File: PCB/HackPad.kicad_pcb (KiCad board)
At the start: 2 copper layers, 61.5 x 94 mm, 34 parts, among them SW1 SW_Push, SW10 RotaryEncoder, SW2 SW_Push, SW3 SW_Push, SW4 SW_Push, SW5 SW_Push, SW6 SW_Push, SW7 SW_Push, SW8 SW_Push, SW9 SW_Push, U1 MOUDLE-SEEEDUINO-XIAO, U2 ER_OLEDM0.91_1x-I2C

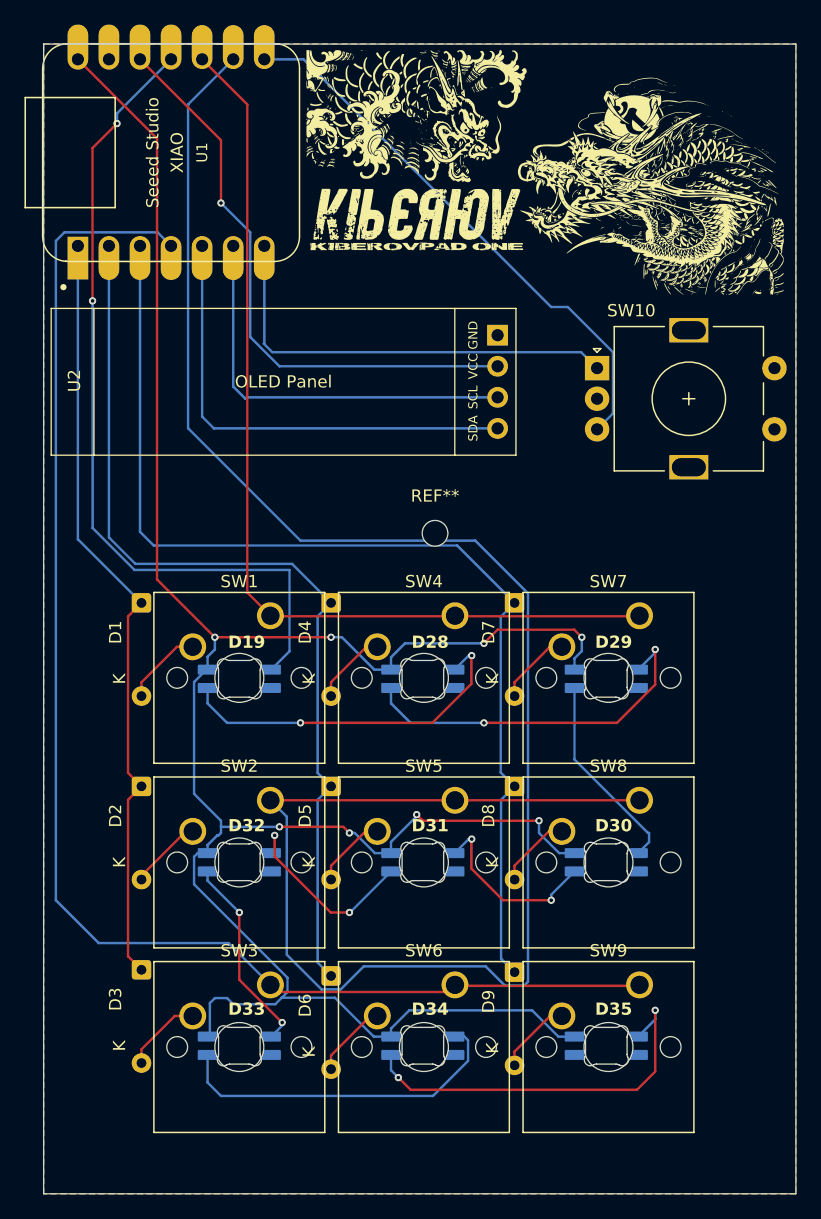
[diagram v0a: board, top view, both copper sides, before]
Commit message: changed pcb design
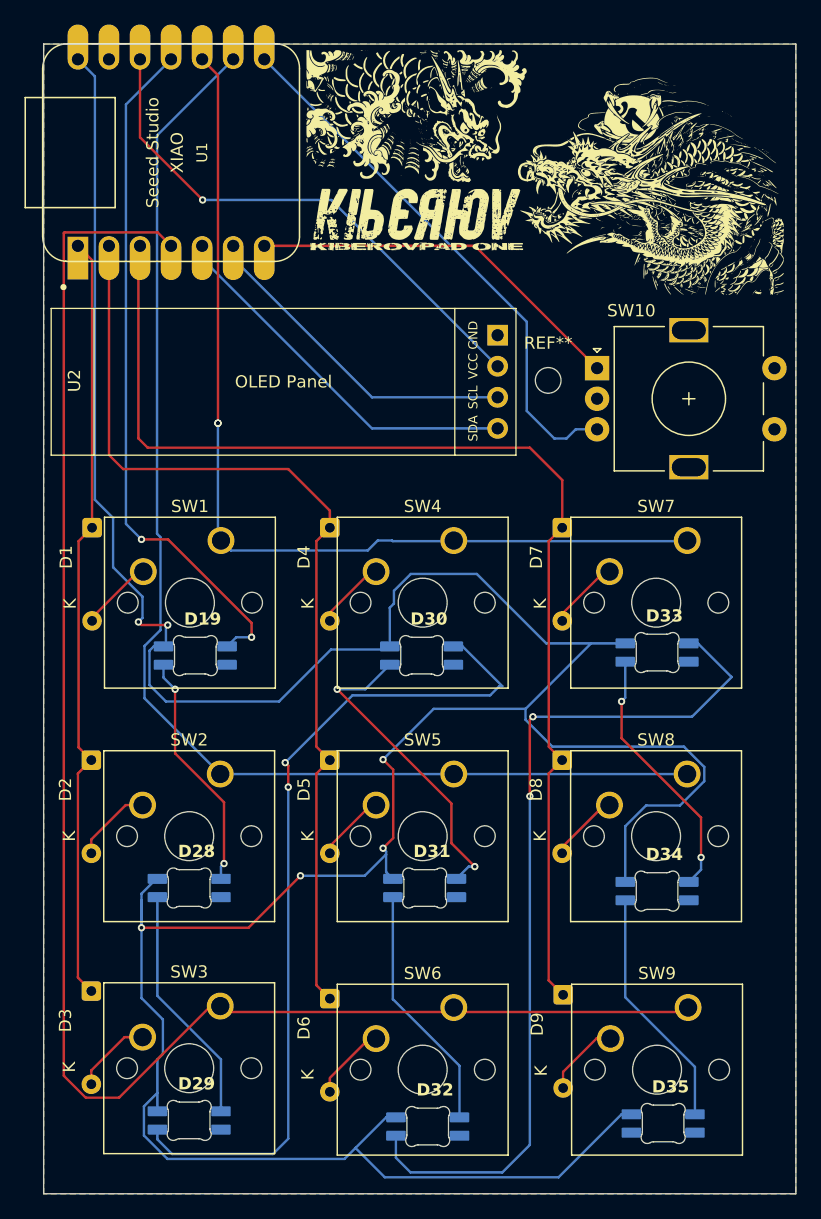
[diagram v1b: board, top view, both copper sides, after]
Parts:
- moved D29 49.7 mm to (135.9, 124.1)
- moved D33 46.9 mm to (174.1, 85.9)
- moved D32 26.5 mm to (155.4, 124.6)
- moved D28 25.6 mm to (135.9, 105.1)
- moved D34 22.9 mm to (174.1, 105.4)
- moved D30 22.7 mm to (154.9, 86.1)
- moved REF** 15.6 mm to (165.2, 63.5)
- moved D35 7.87 mm to (174.6, 124.4)
- moved D1 7.36 mm to (128.0, 75.5)
- moved SW1 7.36 mm to (138.5, 76.6)
- moved D7 7.28 mm to (166.4, 75.5)
- moved SW7 7.28 mm to (176.6, 76.6)
- moved D4 6.15 mm to (147.4, 75.5)
- moved SW4 6.15 mm to (157.5, 76.6)
- moved D2 4.63 mm to (127.9, 94.5)
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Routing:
- net +5V: track 194.3 -> 265.6 mm, vias 8 -> 6
- net coloumn1: track 162.6 -> 102.4 mm
- net Net-(D32-DOUT): track 16.4 -> 71.5 mm
- net Net-(D29-DOUT): track 16.5 -> 69.1 mm, vias 0 -> 2
- net coloumn0: track 115.2 -> 133.4 mm
- net Net-(D34-DOUT): track 31.9 -> 19.9 mm, vias 2 -> 0
- net Net-(D30-DOUT): track 15.0 -> 26.2 mm
- net LED: track 67.3 -> 56.6 mm
- net Net-(D28-DOUT): track 29.9 -> 19.7 mm, vias 2 -> 0
- net Net-(D19-DOUT): track 29.0 -> 19.7 mm
- net SDA: track 38.5 -> 30.9 mm
- net row2: track 88.4 -> 95.8 mm
- net Net-(D33-DOUT): track 28.1 -> 21.2 mm, vias 0 -> 2
- net SCL: track 33.6 -> 27.4 mm
- net encoderA: track 36.1 -> 31.4 mm, vias 0 -> 1
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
